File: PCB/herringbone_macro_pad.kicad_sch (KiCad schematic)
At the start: 33 parts, among them J1 Screw_Terminal_01x04, SW1 CherryMX_2.75u_PCB_StabWireBo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, SW10 CherryMX_1.00u_PCB, SW11 SW_Push, SW2 CherryMX_1.00u_PCB, SW3 CherryMX_2.75u_PCB_StabWireBo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, SW4 CherryMX_2.75u_PCB_StabWireBo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, SW5 CherryMX_1.00u_PCB, SW6 CherryMX_2.75u_PCB_StabWireBo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, SW7 CherryMX_2.75u_PCB_StabWireBo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, SW8 CherryMX_1.00u_PCB, SW9 CherryMX_2.75u_PCB_StabWireBo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, U1 SRV05-4, U2 AMS1117, U3 STM32L151C8TxA, Y1 Crystal

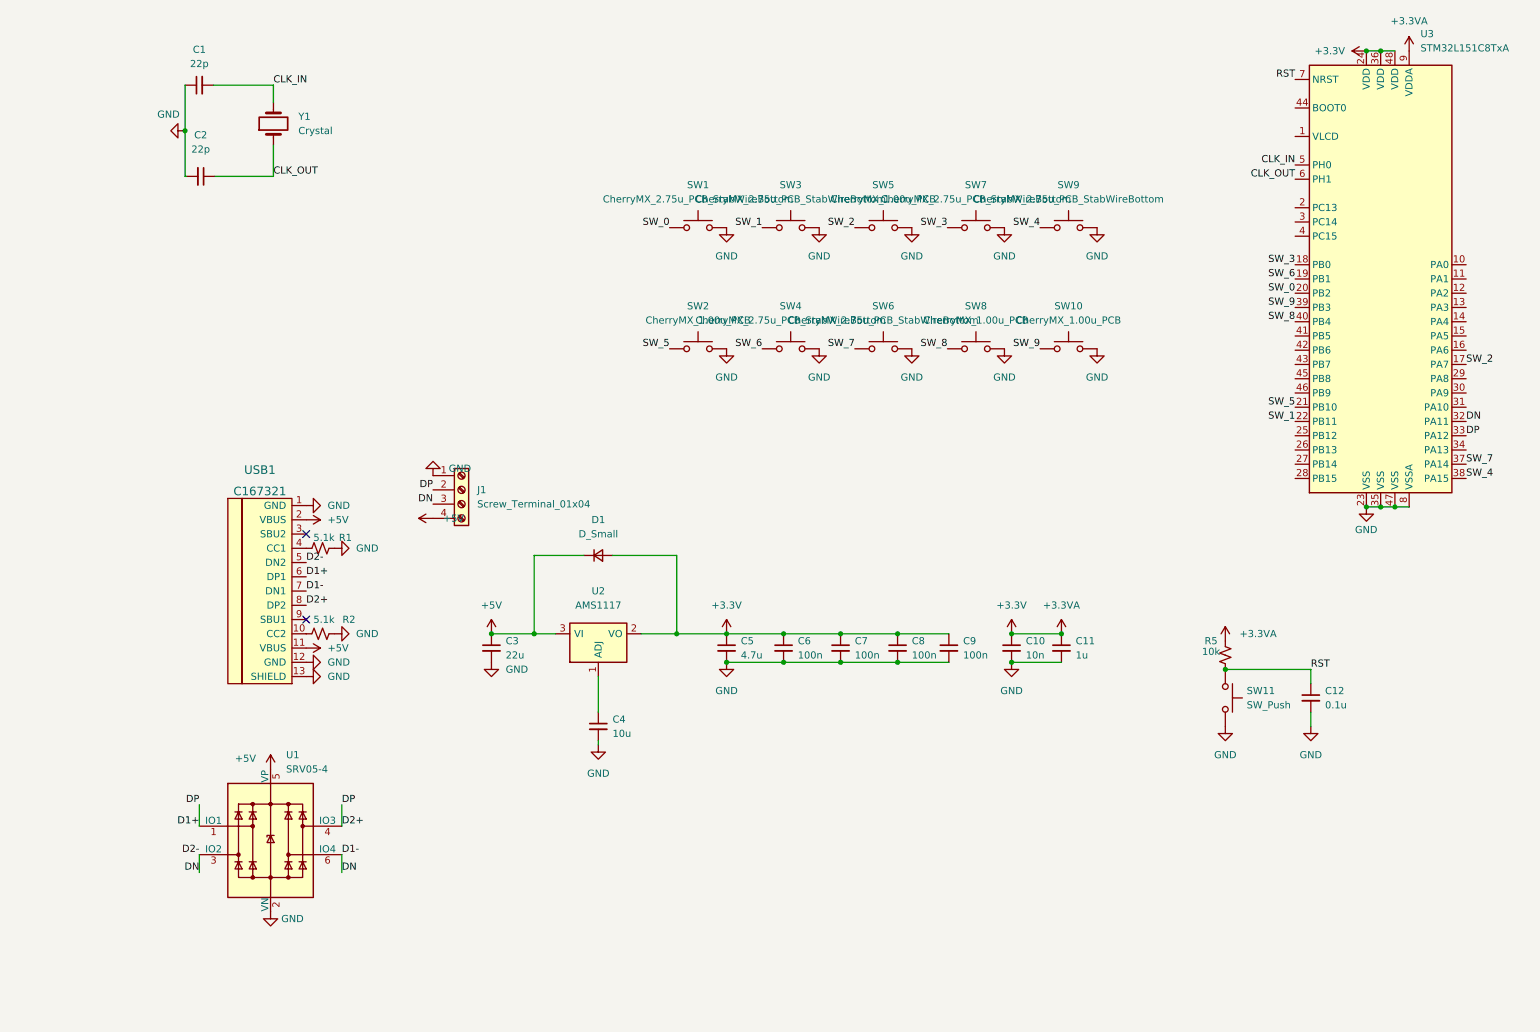
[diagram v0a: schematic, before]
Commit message: Hardware revision.
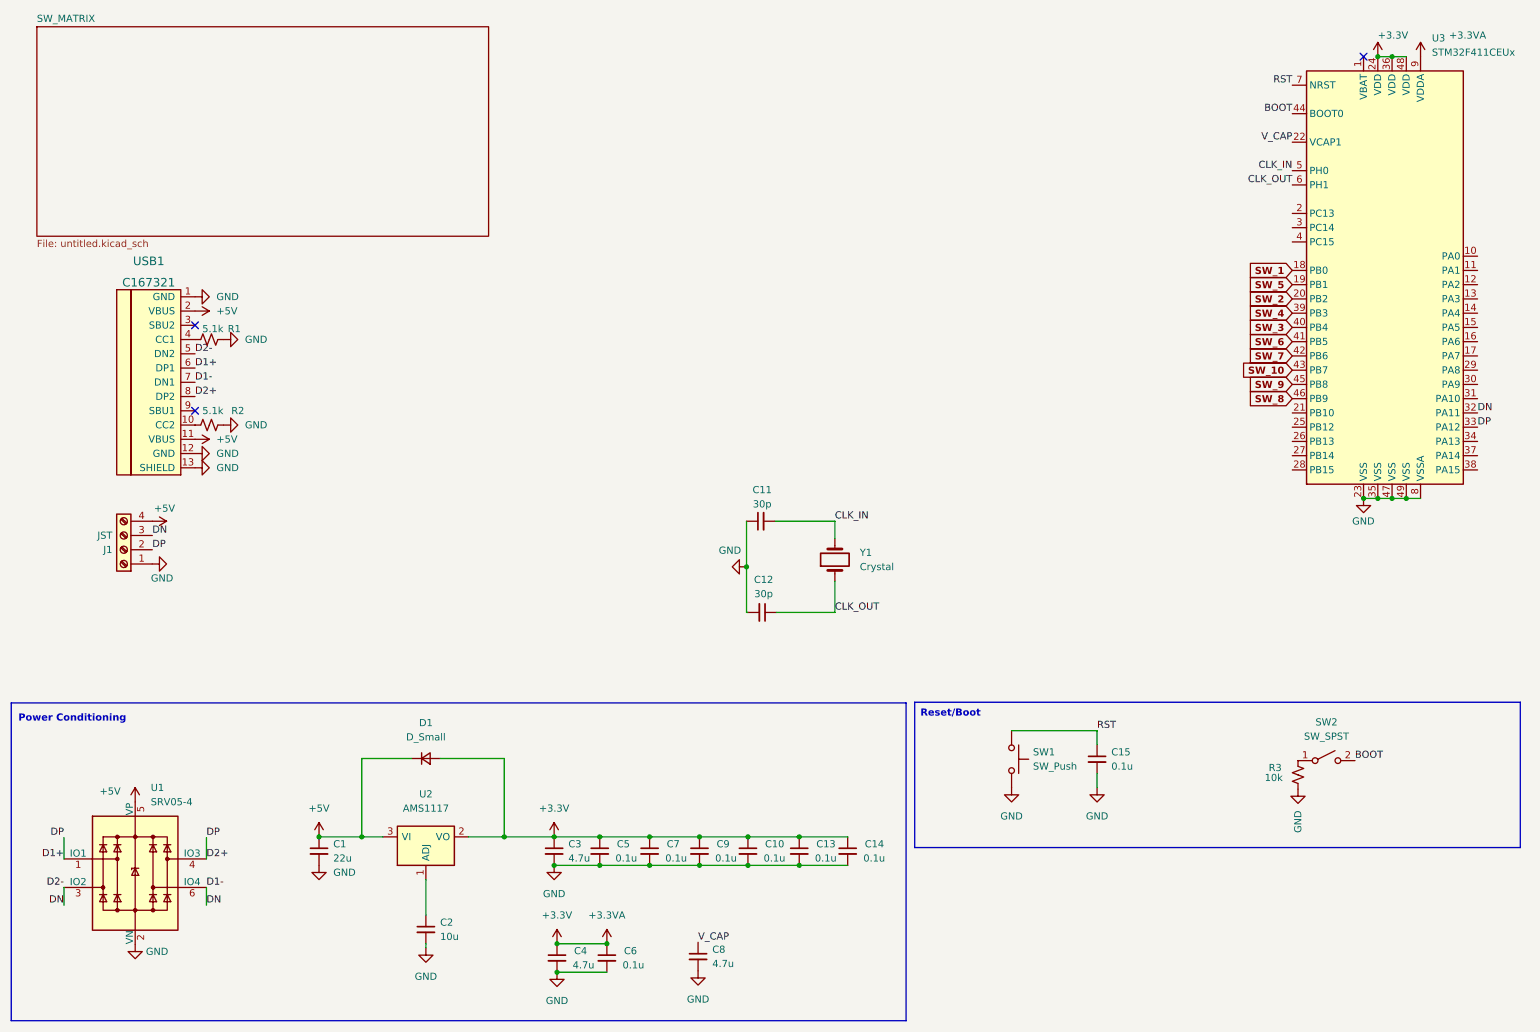
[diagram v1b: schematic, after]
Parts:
- removed C11: 1u, Keebio-Parts:C_0603, symbol Device:C_Small
- removed R5: 10k, Keebio-Parts:R_0603, symbol Device:R_Small_US
- removed SW1, SW3, SW4, SW6, SW7, SW9: CherryMX_2.75u_PCB_StabWireBottom, CherryMX_PCB_StabWireBottom:CherryMX_2.75u_PCB_StabWireBottom, symbol Switch:SW_Push
- removed SW10, SW2, SW5, SW8: CherryMX_1.00u_PCB, CherryMX_PCB:CherryMX_1.00u_PCB, symbol Switch:SW_Push
- removed U3: STM32L151C8TxA, Package_QFP:LQFP-48_7x7mm_P0.5mm, symbol MCU_ST_STM32L1:STM32L151C8TxA
- added C13, C14: 0.1u, Keebio-Parts:C_0402, symbol Device:C_Small
- added C3, C4: 4.7u, Keebio-Parts:C_0402, symbol Device:C_Small
- added R3: 10k, Keebio-Parts:R_0402, symbol Device:R_Small_US
- added SW2: SW_SPST, Button_Switch_SMD:SW_SPDT_PCM12, symbol Switch:SW_SPST
- added U3: STM32F411CEUx, Package_DFN_QFN:QFN-48-1EP_7x7mm_P0.5mm_EP5.6x5.6mm, symbol MCU_ST_STM32F4:STM32F411CEUx
- C1: renamed from C3; footprint Keebio-Parts:C_0603 -> Keebio-Parts:C_0402
- C10: value 10n -> 0.1u; footprint Keebio-Parts:C_0603 -> Keebio-Parts:C_0402
- C11: renamed from C1; value 22p -> 30p; footprint Keebio-Parts:C_0603 -> Keebio-Parts:C_0402
- C12: renamed from C2; value 22p -> 30p; footprint Keebio-Parts:C_0603 -> Keebio-Parts:C_0402
- C15: renamed from C12; footprint Keebio-Parts:C_0603 -> Keebio-Parts:C_0402
- C2: renamed from C4; footprint Keebio-Parts:C_0603 -> Keebio-Parts:C_0402
- C5: value 4.7u -> 0.1u; footprint Keebio-Parts:C_0603 -> Keebio-Parts:C_0402
- C6, C7, C9: value 100n -> 0.1u; footprint Keebio-Parts:C_0603 -> Keebio-Parts:C_0402
- C8: value 100n -> 4.7u; footprint Keebio-Parts:C_0603 -> Keebio-Parts:C_0402
- J1: value Screw_Terminal_01x04 -> JST
- R1, R2: footprint Keebio-Parts:R_0603 -> Keebio-Parts:R_0402
- renumbered SW11 to SW1
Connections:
- net +3.3VA: now also C13.1, C14.1, C3.1, C4.1, U3.24 (VDD), U3.36 (VDD), U3.48 (VDD), U3.9 (VDDA); no longer C8.1
- net CLK_IN: now also U3.5 (PH0)
- net CLK_OUT: now also U3.6 (PH1)
- net D1+: now also U3.33 (PA12)
- net D1-: now also U3.32 (PA11)
- net GND: now also C13.2, C14.2, C3.2, C4.2, R3.1, U3.23 (VSS), U3.35 (VSS), U3.47 (VSS), U3.49 (VSS), U3.8 (VSSA)
- net RST: now also U3.7 (NRST)
- net SW_1: now also U3.18 (PB0)
- net SW_2: now also U3.20 (PB2)
- net SW_3: now also U3.40 (PB4)
- net SW_4: now also U3.39 (PB3)
- net SW_5: now also U3.19 (PB1)
- net SW_6: now also U3.41 (PB5)
- net SW_7: now also U3.42 (PB6)
- net SW_8: now also U3.46 (PB9)
- net SW_9: now also U3.45 (PB8)
- new net: R3.2, SW2.1 (A)
- new net BOOT: SW2.2 (B), U3.44 (BOOT0)
- new net SW_10: U3.43 (PB7)
- new net V_CAP: C8.1, U3.22 (VCAP1)
- no-connect marks 2 -> 3
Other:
- added sheet SW_MATRIX (untitled.kicad_sch)
- note added: "Power Conditioning"
- note added: "Reset/Boot"
- moved on the sheet: C1, C11, C12, C15, C2, D1, J1, R1, R2, SW1, U1, U2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
